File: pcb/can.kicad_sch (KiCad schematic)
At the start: 27 parts, among them J3 C-OBD-II-16M, J4 GND_Connect, U6 TCAN337, U7 LM2842X, U8 LM66100DCK

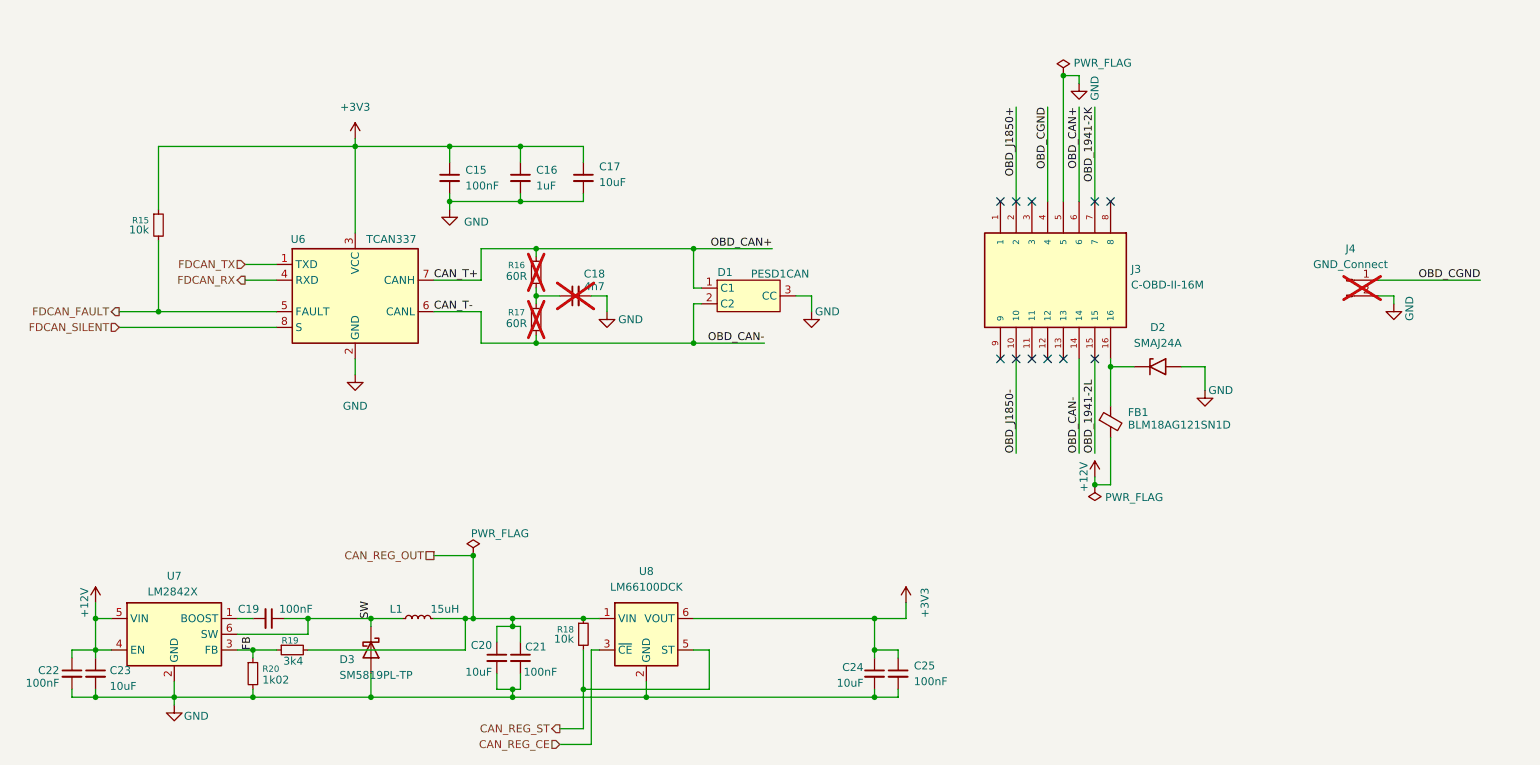
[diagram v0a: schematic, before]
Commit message: update
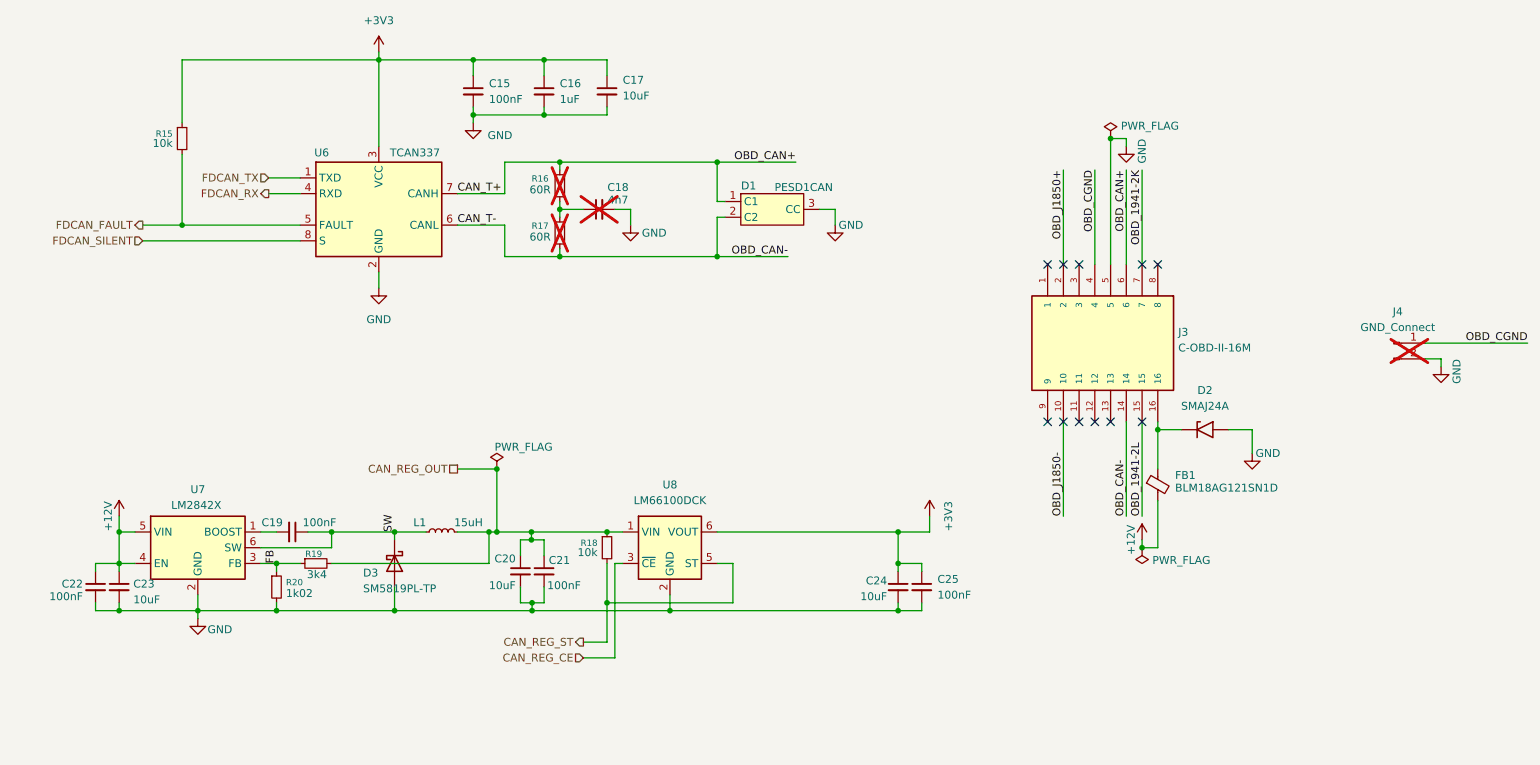
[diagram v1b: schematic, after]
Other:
- moved on the sheet: C15, C16, C17, C18, C19, C20, C21, C22, C23, C24, C25, D1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
